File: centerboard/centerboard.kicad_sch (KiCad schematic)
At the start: 2 parts, among them SW1 SW_Push, U1 ProMicro

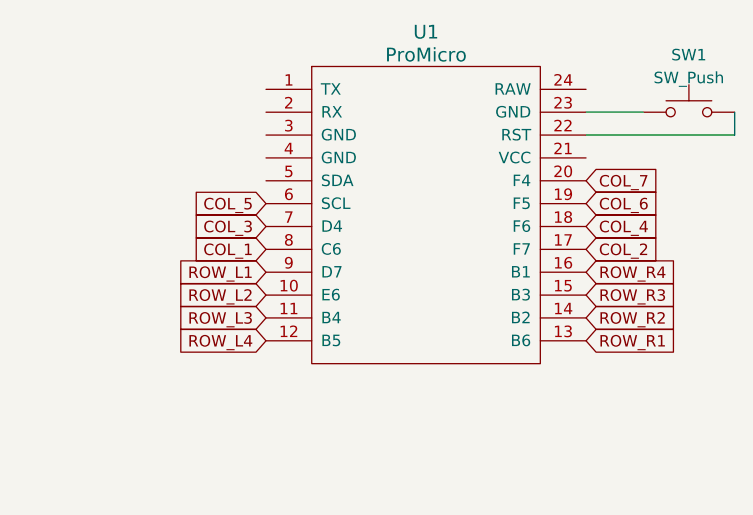
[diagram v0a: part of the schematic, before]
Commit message: centerboard redone, in 1.0 form I think
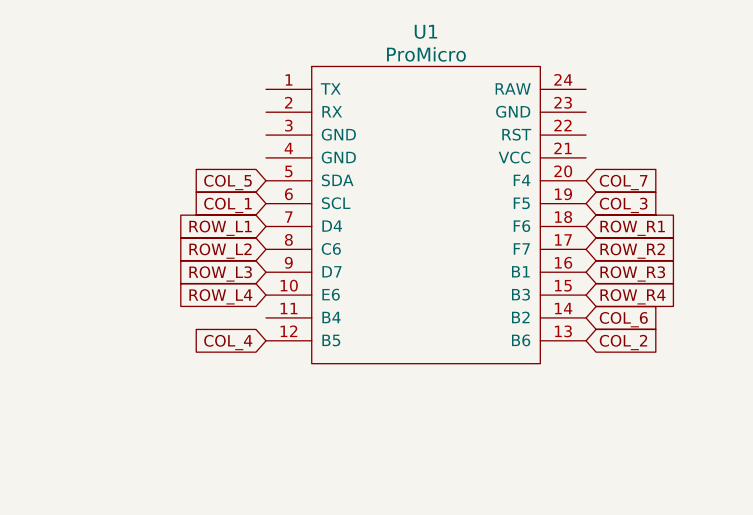
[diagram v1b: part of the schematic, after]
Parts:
- removed SW1: SW_Push, Button_Switch_THT:SW_PUSH_6mm, symbol Switch:SW_Push
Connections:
- net COL_1: now also U1.6 (SCL); no longer U1.8 (C6)
- net COL_2: now also U1.13 (B6); no longer U1.17 (F7)
- net COL_3: now also U1.19 (F5); no longer U1.7 (D4)
- net COL_4: now also U1.12 (B5); no longer U1.18 (F6)
- net COL_5: now also U1.5 (SDA); no longer U1.6 (SCL)
- net COL_6: now also U1.14 (B2); no longer U1.19 (F5)
- net ROW_L1: now also U1.7 (D4); no longer U1.9 (D7)
- net ROW_L2: now also U1.8 (C6); no longer U1.10 (E6)
- net ROW_L3: now also U1.9 (D7); no longer U1.11 (B4)
- net ROW_L4: now also U1.10 (E6); no longer U1.12 (B5)
- net ROW_R1: now also U1.18 (F6); no longer U1.13 (B6)
- net ROW_R2: now also U1.17 (F7); no longer U1.14 (B2)
- net ROW_R3: now also U1.16 (B1); no longer U1.15 (B3)
- net ROW_R4: now also U1.15 (B3); no longer U1.16 (B1)
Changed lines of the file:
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@@
 (kicad_sch (version 20230121) (generator eeschema)
   (paper "A4")
-  (wire (pts (xy 222.25 54.61) (xy 205.74 54.61))
-    (stroke (width 0) (type default))
-  )
-  (wire (pts (xy 222.25 52.07) (xy 222.25 54.61))
-    (stroke (width 0) (type default))
-  )
-  (wire (pts (xy 205.74 52.07) (xy 212.09 52.07))
-    (stroke (width 0) (type default))
-  )
   (global_label "COL_7" (shape input) (at 205.74 59.69 0) (fields_autoplaced)
     (effects (font (size 1.27 1.27)) (justify left))
@@
     )
   )
-  (global_label "ROW_R1" (shape input) (at 205.74 77.47 0) (fields_autoplaced)
+  (global_label "ROW_R1" (shape input) (at 205.74 64.77 0) (fields_autoplaced)
     (effects (font (size 1.27 1.27)) (justify left))
-    (property "Intersheetrefs" "${INTERSHEET_REFS}" (at 216.1448 77.47 0)
+    (property "Intersheetrefs" "${INTERSHEET_REFS}" (at 216.1448 64.77 0)
       (effects (font (size 1.27 1.27)) (justify left) hide)
     )
   )
-  (global_label "ROW_R2" (shape input) (at 205.74 74.93 0) (fields_autoplaced)
+  (global_label "ROW_R2" (shape input) (at 205.74 67.31 0) (fields_autoplaced)
     (effects (font (size 1.27 1.27)) (justify left))
-    (property "Intersheetrefs" "${INTERSHEET_REFS}" (at 216.1448 74.93 0)
+    (property "Intersheetrefs" "${INTERSHEET_REFS}" (at 216.1448 67.31 0)
       (effects (font (size 1.27 1.27)) (justify left) hide)
     )
@@
     )
   )
-  (global_label "COL_6" (shape input) (at 205.74 62.23 0) (fields_autoplaced)
+  (global_label "COL_6" (shape input) (at 205.74 74.93 0) (fields_autoplaced)
     (effects (font (size 1.27 1.27)) (justify left))
-    (property "Intersheetrefs" "${INTERSHEET_REFS}" (at 214.4515 62.23 0)
+    (property "Intersheetrefs" "${INTERSHEET_REFS}" (at 214.4515 74.93 0)
       (effects (font (size 1.27 1.27)) (justify left) hide)
     )
@@
     )
   )
-  (global_label "COL_1" (shape input) (at 170.18 67.31 180) (fields_autoplaced)
-    (effects (font (size 1.27 1.27)) (justify right))
-    (property "Intersheetrefs" "${INTERSHEET_REFS}" (at 161.4685 67.31 0)
-      (effects (font (size 1.27 1.27)) (justify right) hide)
-    )
-  )
-  (global_label "COL_5" (shape input) (at 170.18 62.23 180) (fields_autoplaced)
+  (global_label "COL_1" (shape input) (at 170.18 62.23 180) (fields_autoplaced)
     (effects (font (size 1.27 1.27)) (justify right))
     (property "Intersheetrefs" "${INTERSHEET_REFS}" (at 161.4685 62.23 0)
@@
     )
   )
-  (global_label "COL_2" (shape input) (at 205.74 67.31 0) (fields_autoplaced)
+  (global_label "COL_5" (shape input) (at 170.18 59.69 180) (fields_autoplaced)
+    (effects (font (size 1.27 1.27)) (justify right))
+    (property "Intersheetrefs" "${INTERSHEET_REFS}" (at 161.4685 59.69 0)
+      (effects (font (size 1.27 1.27)) (justify right) hide)
+    )
+  )
+  (global_label "COL_2" (shape input) (at 205.74 77.47 0) (fields_autoplaced)
     (effects (font (size 1.27 1.27)) (justify left))
-    (property "Intersheetrefs" "${INTERSHEET_REFS}" (at 214.4515 67.31 0)
+    (property "Intersheetrefs" "${INTERSHEET_REFS}" (at 214.4515 77.47 0)
       (effects (font (size 1.27 1.27)) (justify left) hide)
     )
   )
-  (global_label "COL_3" (shape input) (at 170.18 64.77 180) (fields_autoplaced)
-    (effects (font (size 1.27 1.27)) (justify right))
-    (property "Intersheetrefs" "${INTERSHEET_REFS}" (at 161.4685 64.77 0)
-      (effects (font (size 1.27 1.27)) (justify right) hide)
+  (global_label "COL_3" (shape input) (at 205.74 62.23 0) (fields_autoplaced)
+    (effects (font (size 1.27 1.27)) (justify left))
+    (property "Intersheetrefs" "${INTERSHEET_REFS}" (at 214.4515 62.23 0)
+      (effects (font (size 1.27 1.27)) (justify left) hide)
     )
   )
@@
     )
   )
-  (global_label "ROW_R4" (shape input) (at 205.74 69.85 0) (fields_autoplaced)
+  (global_label "ROW_R4" (shape input) (at 205.74 72.39 0) (fields_autoplaced)
     (effects (font (size 1.27 1.27)) (justify left))
-    (property "Intersheetrefs" "${INTERSHEET_REFS}" (at 216.1448 69.85 0)
+    (property "Intersheetrefs" "${INTERSHEET_REFS}" (at 216.1448 72.39 0)
       (effects (font (size 1.27 1.27)) (justify left) hide)
     )
   )
-  (global_label "ROW_L4" (shape input) (at 170.18 77.47 180) (fields_autoplaced)
+  (global_label "ROW_L4" (shape input) (at 170.18 72.39 180) (fields_autoplaced)
     (effects (font (size 1.27 1.27)) (justify right))
-    (property "Intersheetrefs" "${INTERSHEET_REFS}" (at 160.0171 77.47 0)
+    (property "Intersheetrefs" "${INTERSHEET_REFS}" (at 160.0171 72.39 0)
       (effects (font (size 1.27 1.27)) (justify right) hide)
     )
@@
     )
   )
-  (global_label "COL_4" (shape input) (at 205.74 64.77 0) (fields_autoplaced)
-    (effects (font (size 1.27 1.27)) (justify left))
-    (property "Intersheetrefs" "${INTERSHEET_REFS}" (at 214.4515 64.77 0)
-      (effects (font (size 1.27 1.27)) (justify left) hide)
+  (global_label "COL_4" (shape input) (at 170.18 77.47 180) (fields_autoplaced)
+    (effects (font (size 1.27 1.27)) (justify right))
+    (property "Intersheetrefs" "${INTERSHEET_REFS}" (at 161.4685 77.47 0)
+      (effects (font (size 1.27 1.27)) (justify right) hide)
     )
   )
-  (global_label "ROW_L2" (shape input) (at 170.18 72.39 180) (fields_autoplaced)
+  (global_label "ROW_L2" (shape input) (at 170.18 67.31 180) (fields_autoplaced)
     (effects (font (size 1.27 1.27)) (justify right))
-    (property "Intersheetrefs" "${INTERSHEET_REFS}" (at 160.0171 72.39 0)
+    (property "Intersheetrefs" "${INTERSHEET_REFS}" (at 160.0171 67.31 0)
       (effects (font (size 1.27 1.27)) (justify right) hide)
     )
@@
     )
   )
-  (global_label "ROW_L1" (shape input) (at 170.18 69.85 180) (fields_autoplaced)
+  (global_label "ROW_L1" (shape input) (at 170.18 64.77 180) (fields_autoplaced)
     (effects (font (size 1.27 1.27)) (justify right))
-    (property "Intersheetrefs" "${INTERSHEET_REFS}" (at 160.0171 69.85 0)
+    (property "Intersheetrefs" "${INTERSHEET_REFS}" (at 160.0171 64.77 0)
       (effects (font (size 1.27 1.27)) (justify right) hide)
     )
   )
-  (global_label "ROW_R3" (shape input) (at 205.74 72.39 0) (fields_autoplaced)
+  (global_label "ROW_R3" (shape input) (at 205.74 69.85 0) (fields_autoplaced)
     (effects (font (size 1.27 1.27)) (justify left))
-    (property "Intersheetrefs" "${INTERSHEET_REFS}" (at 216.1448 72.39 0)
+    (property "Intersheetrefs" "${INTERSHEET_REFS}" (at 216.1448 69.85 0)
       (effects (font (size 1.27 1.27)) (justify left) hide)
     )
@@
     )
   )
-  (global_label "ROW_L3" (shape input) (at 170.18 74.93 180) (fields_autoplaced)
+  (global_label "ROW_L3" (shape input) (at 170.18 69.85 180) (fields_autoplaced)
     (effects (font (size 1.27 1.27)) (justify right))
-    (property "Intersheetrefs" "${INTERSHEET_REFS}" (at 160.0171 74.93 0)
+    (property "Intersheetrefs" "${INTERSHEET_REFS}" (at 160.0171 69.85 0)
       (effects (font (size 1.27 1.27)) (justify right) hide)
     )
@@
         )
       )
-    )
-  )
-  (symbol (lib_id "Switch:SW_Push") (at 217.17 52.07 0) (unit 1)
-    (in_bom yes) (on_board yes) (dnp no) (fields_autoplaced)
-    (property "Reference" "SW1" (at 217.17 45.72 0)
-      (effects (font (size 1.27 1.27)))
-    )
-    (property "Value" "SW_Push" (at 217.17 48.26 0)
-      (effects (font (size 1.27 1.27)))
-    )
-    (property "Footprint" "Button_Switch_THT:SW_PUSH_6mm" (at 217.17 46.99 0)
-      (effects (font (size 1.27 1.27)) hide)
-    )
-    (property "Datasheet" "~" (at 217.17 46.99 0)
-      (effects (font (size 1.27 1.27)) hide)
-    )
-    (pin "1")
-    (pin "2")
-    (instances
-      (project "centerboard"
-        (path "/4cf5c873-f5e9-4261-911c-886f387fb0f3"
-          (reference "SW1") (unit 1)
-        )
-      )
